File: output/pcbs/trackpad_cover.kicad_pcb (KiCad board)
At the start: 2 copper layers, 54.1 x 54.1 mm, 4 parts

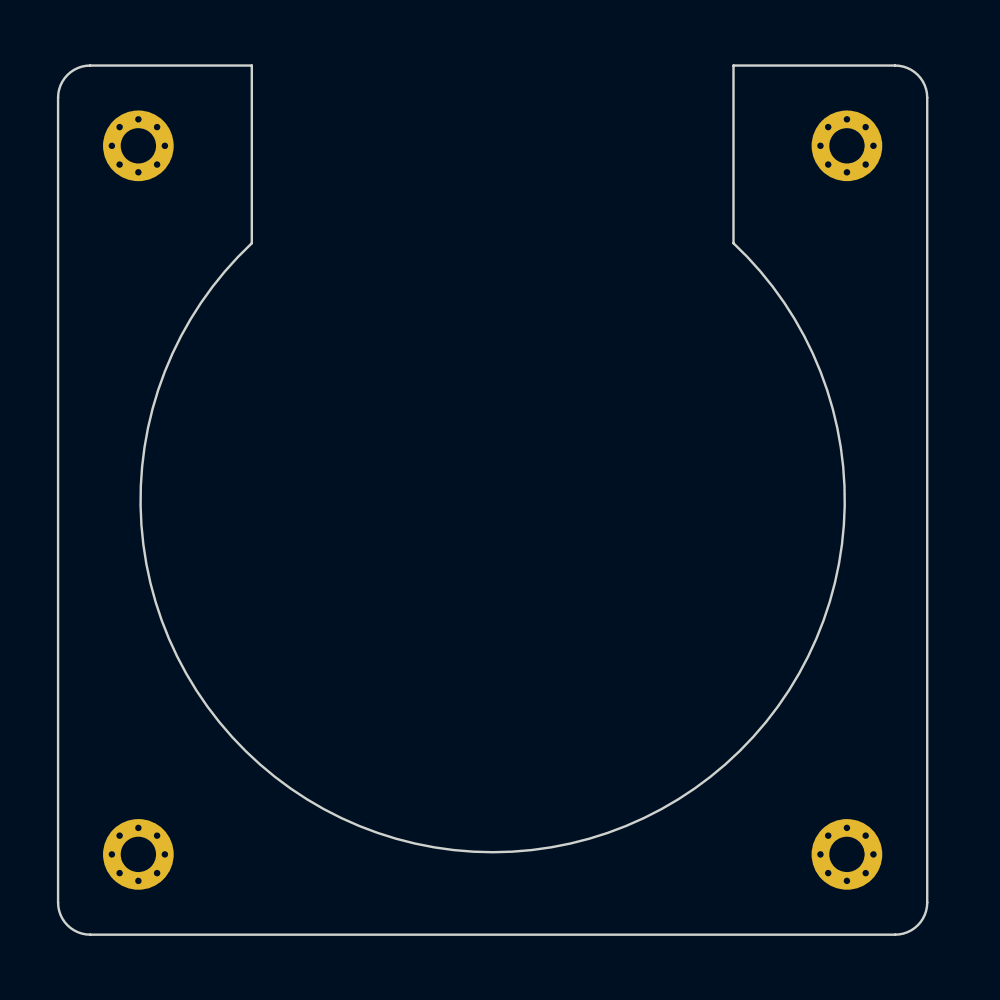
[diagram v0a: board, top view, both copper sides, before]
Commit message: second commit
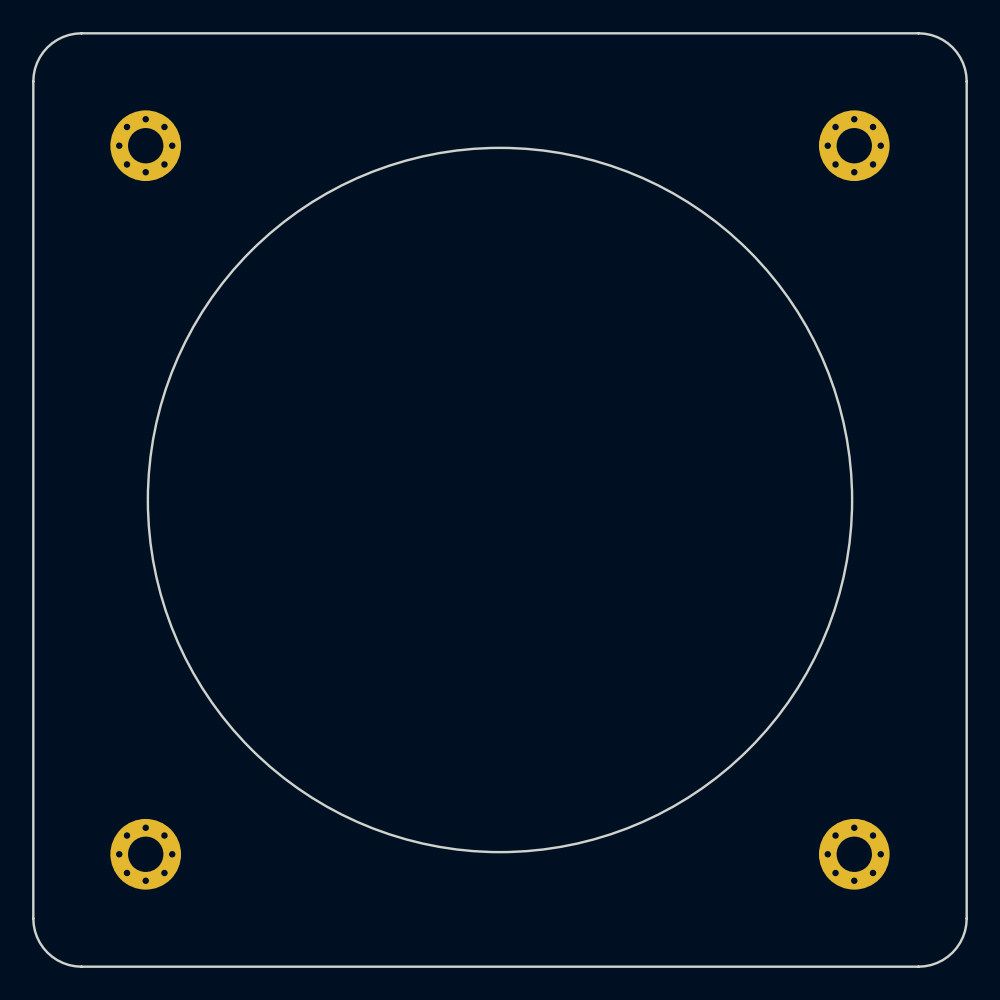
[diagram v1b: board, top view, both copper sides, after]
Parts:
- moved _1 0.46 mm to (227.9, 93.3)
- moved _2 0.46 mm to (183.8, 93.3)
- moved _3 0.46 mm to (227.9, 137.4)
- moved _4 0.46 mm to (183.8, 137.4)
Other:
- board size 54.1 x 54.1 mm -> 58.1 x 58.1 mm
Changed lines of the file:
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@@
   )
     (module "MountingHole_2.2mm_M2_Pad_Via" (version 20210722) (generator pcbnew) (layer "F.Cu")
-      (at 227.4539034 93.2725473 0)
+      (at 227.9113045 93.265776 0)
       (fp_text reference "_1" (at 0 -3.2) (layer "F.SilkS") hide
         (effects (font (size 1 1) (thickness 0.15)))
@@
     )
     (module "MountingHole_2.2mm_M2_Pad_Via" (version 20210722) (generator pcbnew) (layer "F.Cu")
-      (at 183.3239034 93.2725473 0)
+      (at 183.7813045 93.265776 0)
       (fp_text reference "_2" (at 0 -3.2) (layer "F.SilkS") hide
         (effects (font (size 1 1) (thickness 0.15)))
@@
     )
     (module "MountingHole_2.2mm_M2_Pad_Via" (version 20210722) (generator pcbnew) (layer "F.Cu")
-      (at 227.4539034 137.4025473 0)
+      (at 227.9113045 137.395776 0)
       (fp_text reference "_3" (at 0 -3.2) (layer "F.SilkS") hide
         (effects (font (size 1 1) (thickness 0.15)))
@@
     )
     (module "MountingHole_2.2mm_M2_Pad_Via" (version 20210722) (generator pcbnew) (layer "F.Cu")
-      (at 183.3239034 137.4025473 0)
+      (at 183.7813045 137.395776 0)
       (fp_text reference "_4" (at 0 -3.2) (layer "F.SilkS") hide
         (effects (font (size 1 1) (thickness 0.15)))
@@
       (pad "1" thru_hole circle locked (at 0 -1.65) (size 0.7 0.7) (drill 0.4) (layers *.Cu *.Mask))
     )
-  (gr_line (start 180.3239034 142.4025473) (end 230.4539034 142.4025473) (angle 90) (layer Edge.Cuts) (width 0.15))
-(gr_arc (start 230.4539034 140.4025473) (end 230.4539034 142.4025473) (angle -90) (layer Edge.Cuts) (width 0.15))
-(gr_line (start 232.4539034 140.4025473) (end 232.4539034 90.27254730000001) (angle 90) (layer Edge.Cuts) (width 0.15))
-(gr_arc (start 230.4539034 90.27254730000001) (end 232.4539034 90.27254730000001) (angle -90) (layer Edge.Cuts) (width 0.15))
-(gr_line (start 230.4539034 88.27254730000001) (end 220.3889034 88.27254730000001) (angle 90) (layer Edge.Cuts) (width 0.15))
-(gr_line (start 190.3889034 88.27254730000001) (end 180.3239034 88.27254730000001) (angle 90) (layer Edge.Cuts) (width 0.15))
-(gr_arc (start 180.3239034 90.27254730000001) (end 180.3239034 88.27254730000001) (angle -90) (layer Edge.Cuts) (width 0.15))
-(gr_line (start 178.3239034 90.27254730000001) (end 178.3239034 140.4025473) (angle 90) (layer Edge.Cuts) (width 0.15))
-(gr_arc (start 180.3239034 140.4025473) (end 178.3239034 140.4025473) (angle -90) (layer Edge.Cuts) (width 0.15))
-(gr_arc (start 205.3889034 115.3375473) (end 190.3889034 99.3398943) (angle -273.6868327756372) (layer Edge.Cuts) (width 0.15))
-(gr_line (start 220.3889034 99.3398943) (end 220.3889034 88.27254730000001) (angle 90) (layer Edge.Cuts) (width 0.15))
-(gr_line (start 190.3889034 88.27254730000001) (end 190.3889034 99.3398943) (angle 90) (layer Edge.Cuts) (width 0.15))
+  (gr_line (start 179.7813045 144.395776) (end 231.9113045 144.395776) (angle 90) (layer Edge.Cuts) (width 0.15))
+(gr_arc (start 231.9113045 141.395776) (end 231.9113045 144.395776) (angle -90) (layer Edge.Cuts) (width 0.15))
+(gr_line (start 234.9113045 141.395776) (end 234.9113045 89.26577600000002) (angle 90) (layer Edge.Cuts) (width 0.15))
+(gr_arc (start 231.9113045 89.26577600000002) (end 234.9113045 89.26577600000002) (angle -90) (layer Edge.Cuts) (width 0.15))
+(gr_line (start 231.9113045 86.26577600000002) (end 179.7813045 86.26577600000002) (angle 90) (layer Edge.Cuts) (width 0.15))
+(gr_arc (start 179.7813045 89.26577600000002) (end 179.7813045 86.26577600000002) (angle -90) (layer Edge.Cuts) (width 0.15))
+(gr_line (start 176.7813045 89.26577600000002) (end 176.7813045 141.395776) (angle 90) (layer Edge.Cuts) (width 0.15))
+(gr_arc (start 179.7813045 141.395776) (end 176.7813045 141.395776) (angle -90) (layer Edge.Cuts) (width 0.15))
+(gr_circle (center 205.8463045 115.330776) (end 227.7763045 115.330776) (layer Edge.Cuts) (width 0.15))
 )
